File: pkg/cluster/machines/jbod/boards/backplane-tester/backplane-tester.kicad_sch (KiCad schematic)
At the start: 35 parts, among them J1 POWER, J2 BOARD_IN, J3 SAS_OUT, J4 POWER_RES1, J5 POWER_RES2, Q1 N-CH, Q2 P-CH, Q3 P-CH, Q4 N-CH, Q5 N-CH, Q6 N-CH, Q8 N-CH, Q9 N-CH, U1 MCP23008-xSO, U2 NRF52840_ITSY_BITSY

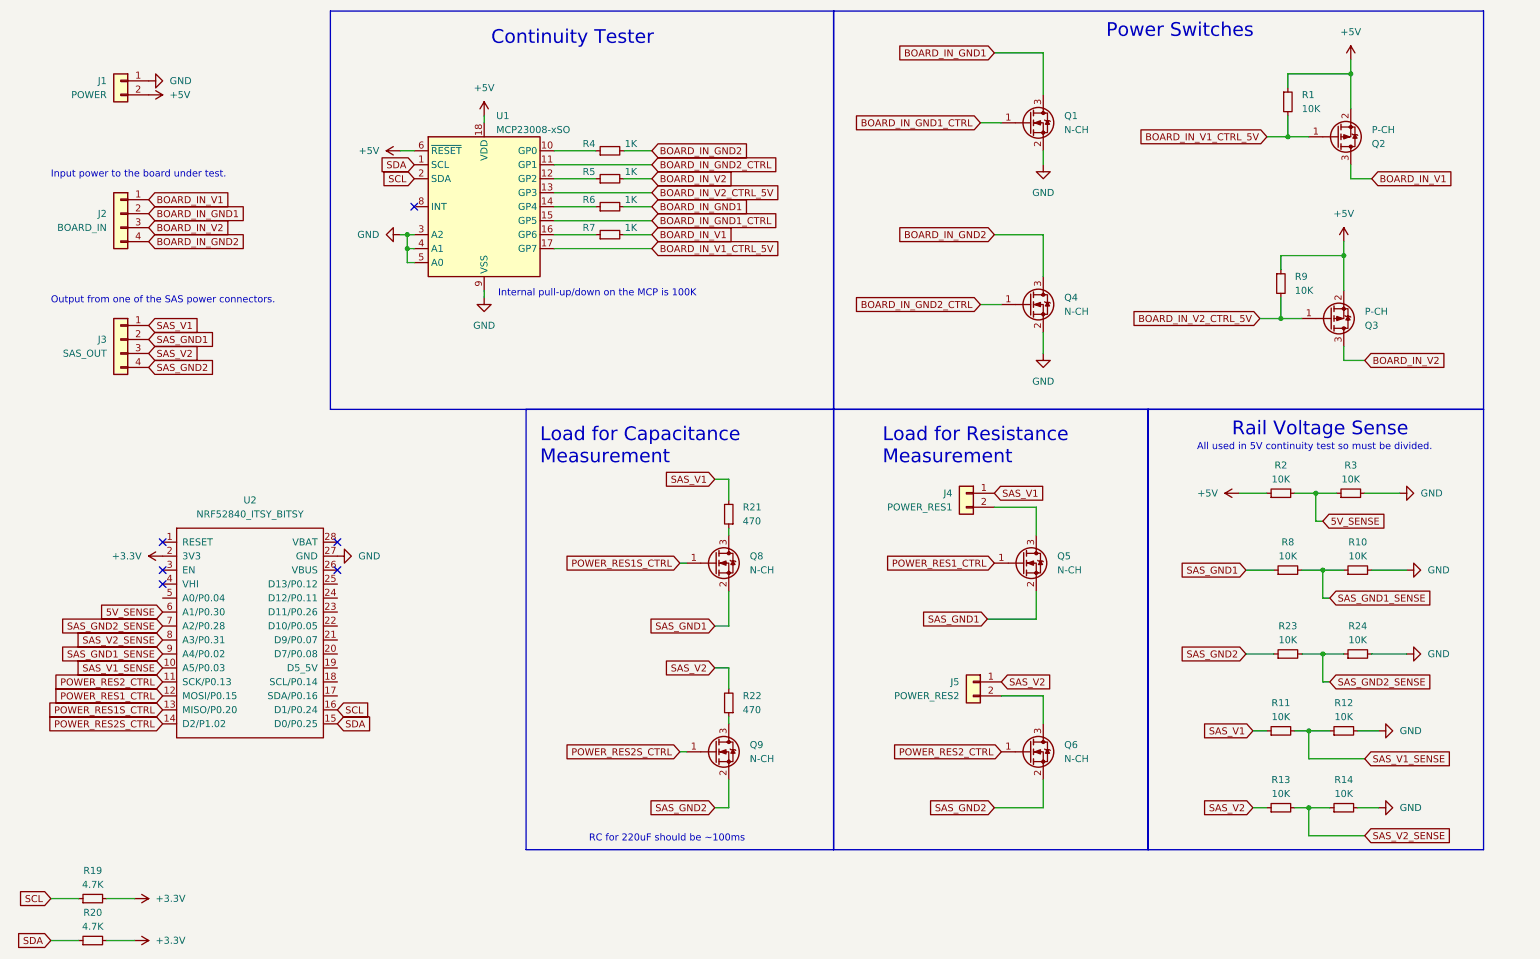
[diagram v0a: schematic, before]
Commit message: Flushing some recent changes.
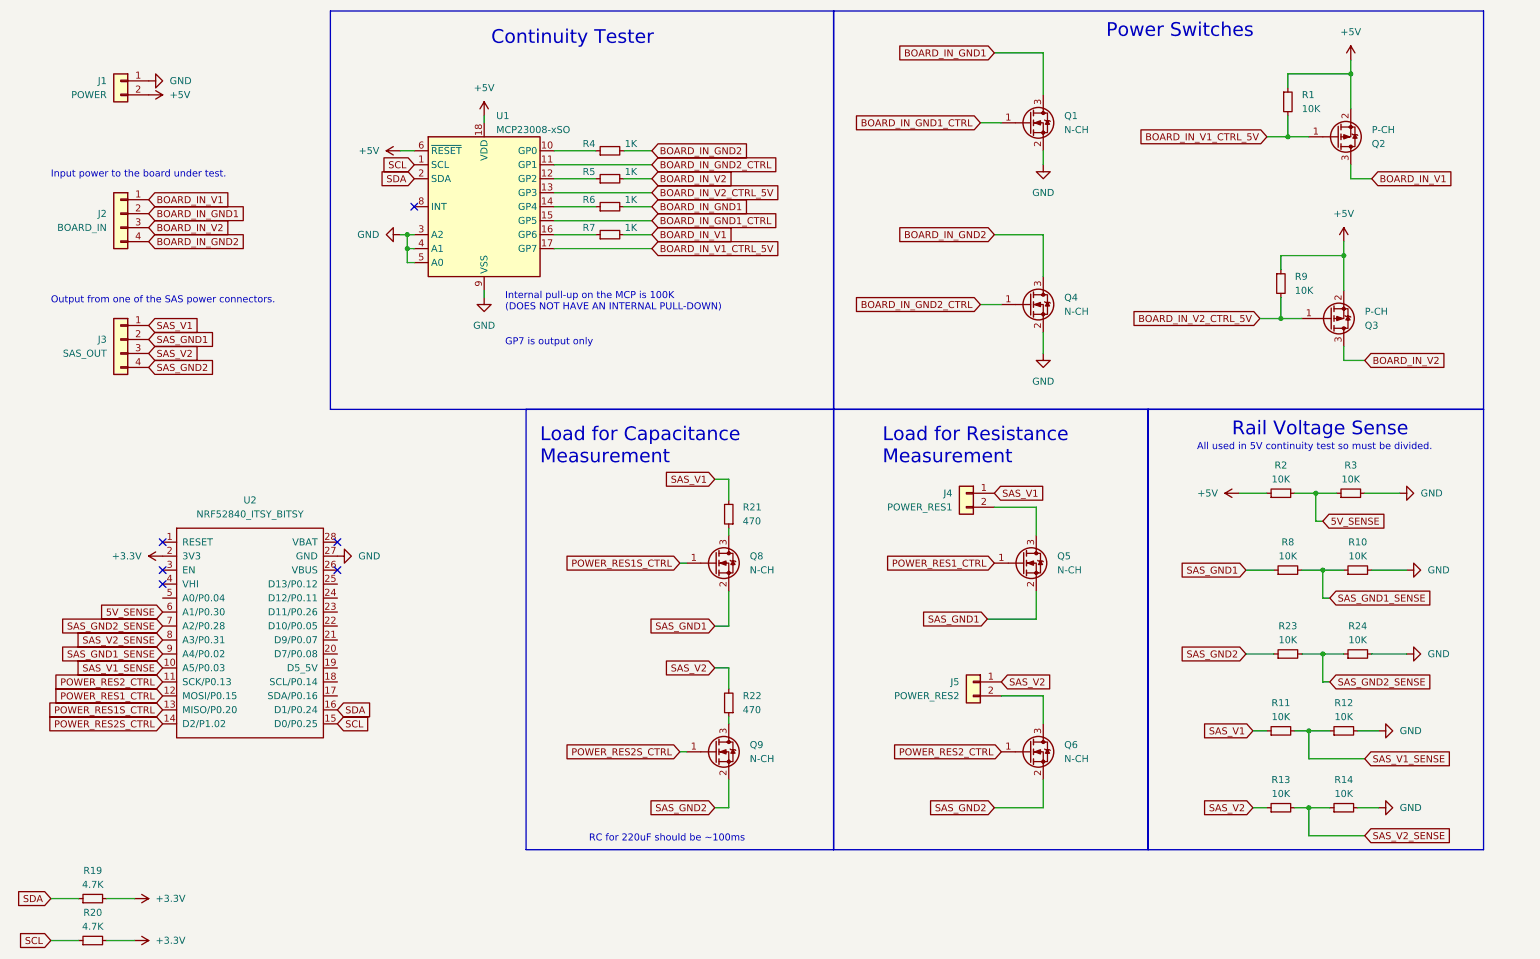
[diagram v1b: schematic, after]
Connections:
- net SCL: now also R20.1, U1.1 (SCL), U2.15 (D0/P0.25); no longer R19.1, U1.2 (SDA), U2.16 (D1/P0.24)
- net SDA: now also R19.1, U1.2 (SDA), U2.16 (D1/P0.24); no longer R20.1, U1.1 (SCL), U2.15 (D0/P0.25)
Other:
- note added: "GP7 is output only"
- note added: "Internal pull-up on the MCP is 100K (DOES NOT HAVE AN INTERNAL PULL-DOWN)"
- note removed: "Internal pull-up/down on the MCP is 100K"
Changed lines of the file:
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@@
     (fill (type none))
   )
-  (text "Internal pull-up/down on the MCP is 100K" (at 105.41 64.77 0)
+  (text "Internal pull-up on the MCP is 100K\n(DOES NOT HAVE AN INTERNAL PULL-DOWN)"
+    (at 106.68 67.31 0)
     (effects (font (size 1.27 1.27)) (justify left bottom))
   )
@@
     (effects (font (size 1.27 1.27)) (justify left bottom))
   )
+  (text "GP7 is output only" (at 106.68 73.66 0)
+    (effects (font (size 1.27 1.27)) (justify left bottom))
+  )
   (text "Load for Resistance\nMeasurement" (at 175.26 95.25 0)
     (effects (font (size 2.5 2.5)) (justify left bottom))
@@
     )
   )
-  (global_label "SDA" (shape input) (at 90.17 40.64 180) (fields_autoplaced)
-    (effects (font (size 1.27 1.27)) (justify right))
-    (property "Intersheetrefs" "${INTERSHEET_REFS}" (at 83.6167 40.64 0)
-      (effects (font (size 1.27 1.27)) (justify right) hide)
-    )
-  )
-  (global_label "SCL" (shape input) (at 90.17 43.18 180) (fields_autoplaced)
-    (effects (font (size 1.27 1.27)) (justify right))
-    (property "Intersheetrefs" "${INTERSHEET_REFS}" (at 83.6772 43.18 0)
+  (global_label "SCL" (shape input) (at 90.17 40.64 180) (fields_autoplaced)
+    (effects (font (size 1.27 1.27)) (justify right))
+    (property "Intersheetrefs" "${INTERSHEET_REFS}" (at 83.6772 40.64 0)
+      (effects (font (size 1.27 1.27)) (justify right) hide)
+    )
+  )
+  (global_label "SDA" (shape input) (at 90.17 43.18 180) (fields_autoplaced)
+    (effects (font (size 1.27 1.27)) (justify right))
+    (property "Intersheetrefs" "${INTERSHEET_REFS}" (at 83.6167 43.18 0)
       (effects (font (size 1.27 1.27)) (justify right) hide)
     )
@@
     )
   )
-  (global_label "SCL" (shape input) (at 76.2 139.7 0) (fields_autoplaced)
-    (effects (font (size 1.27 1.27)) (justify left))
-    (property "Intersheetrefs" "${INTERSHEET_REFS}" (at 82.6928 139.7 0)
+  (global_label "SDA" (shape input) (at 76.2 139.7 0) (fields_autoplaced)
+    (effects (font (size 1.27 1.27)) (justify left))
+    (property "Intersheetrefs" "${INTERSHEET_REFS}" (at 82.7533 139.7 0)
       (effects (font (size 1.27 1.27)) (justify left) hide)
     )
@@
     )
   )
-  (global_label "SCL" (shape input) (at 24.13 173.99 180) (fields_autoplaced)
-    (effects (font (size 1.27 1.27)) (justify right))
-    (property "Intersheetrefs" "${INTERSHEET_REFS}" (at 17.6372 173.99 0)
+  (global_label "SDA" (shape input) (at 24.13 173.99 180) (fields_autoplaced)
+    (effects (font (size 1.27 1.27)) (justify right))
+    (property "Intersheetrefs" "${INTERSHEET_REFS}" (at 17.5767 173.99 0)
       (effects (font (size 1.27 1.27)) (justify right) hide)
     )
@@
     )
   )
-  (global_label "SDA" (shape input) (at 76.2 142.24 0) (fields_autoplaced)
-    (effects (font (size 1.27 1.27)) (justify left))
-    (property "Intersheetrefs" "${INTERSHEET_REFS}" (at 82.7533 142.24 0)
+  (global_label "SCL" (shape input) (at 76.2 142.24 0) (fields_autoplaced)
+    (effects (font (size 1.27 1.27)) (justify left))
+    (property "Intersheetrefs" "${INTERSHEET_REFS}" (at 82.6928 142.24 0)
       (effects (font (size 1.27 1.27)) (justify left) hide)
     )
@@
     )
   )
-  (global_label "SDA" (shape input) (at 24.13 181.61 180) (fields_autoplaced)
-    (effects (font (size 1.27 1.27)) (justify right))
-    (property "Intersheetrefs" "${INTERSHEET_REFS}" (at 17.5767 181.61 0)
-      (effects (font (size 1.27 1.27)) (justify right) hide)
-    )
+  (global_label "SCL" (shape input) (at 24.13 181.61 180) (fields_autoplaced)
+    (effects (font (size 1.27 1.27)) (justify right))
+    (property "Intersheetrefs" "${INTERSHEET_REFS}" (at 17.6372 181.61 0)
+      (effects (font (size 1.27 1.27)) (justify right) hide)
+    )
